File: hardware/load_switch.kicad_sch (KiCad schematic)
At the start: 24 parts, among them Q1 IPT015N10N5, Q2 IPT015N10N5, Q3 IPT015N10N5, Q4 IPT015N10N5, Q5 IPT015N10N5, Q6 IPT015N10N5, Q7 IPT015N10N5, Q8 IPT015N10N5

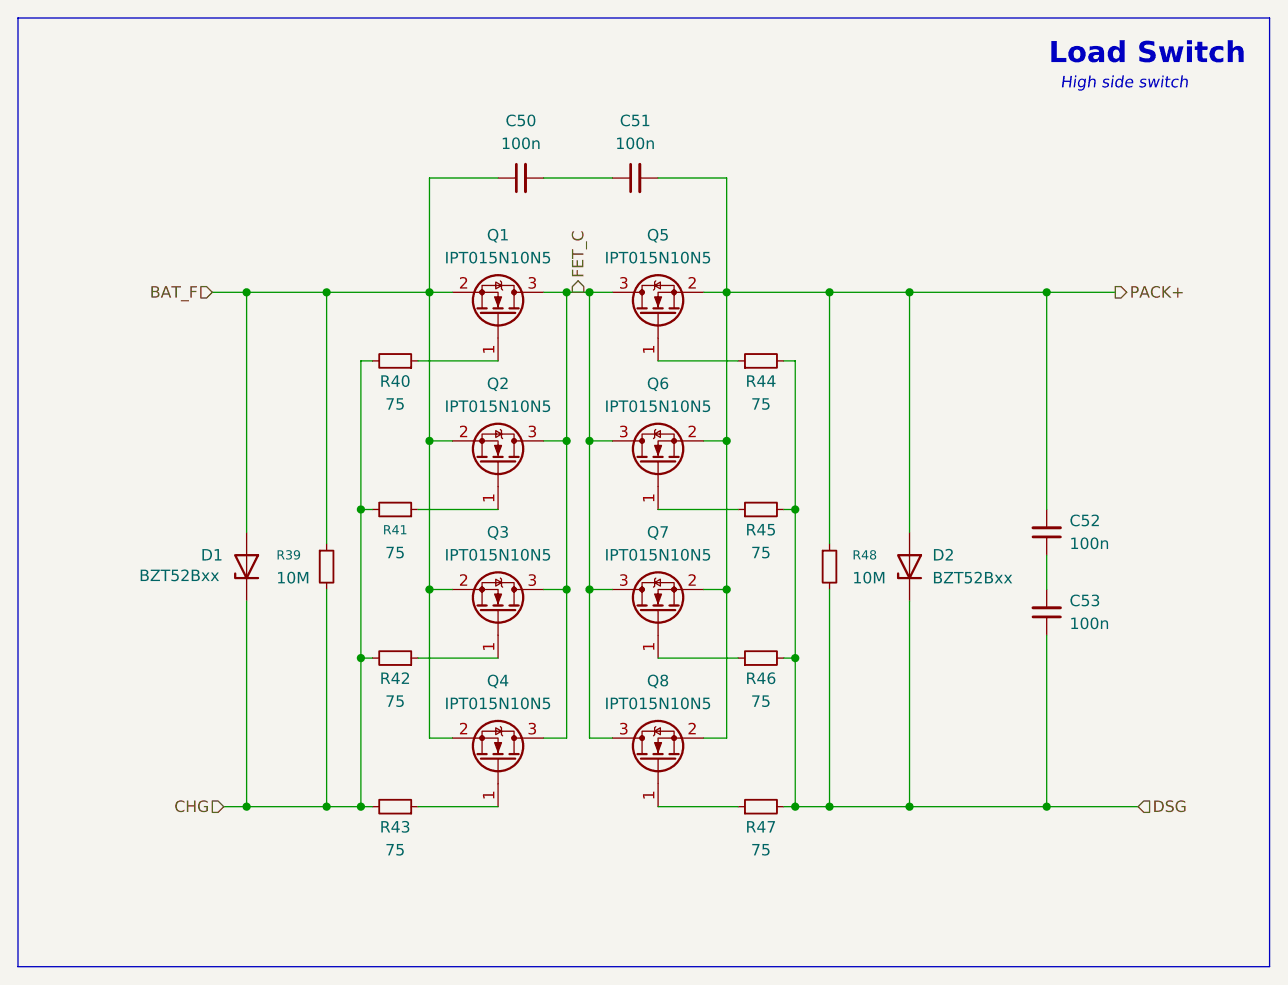
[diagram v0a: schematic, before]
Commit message: Majority of layout placement done
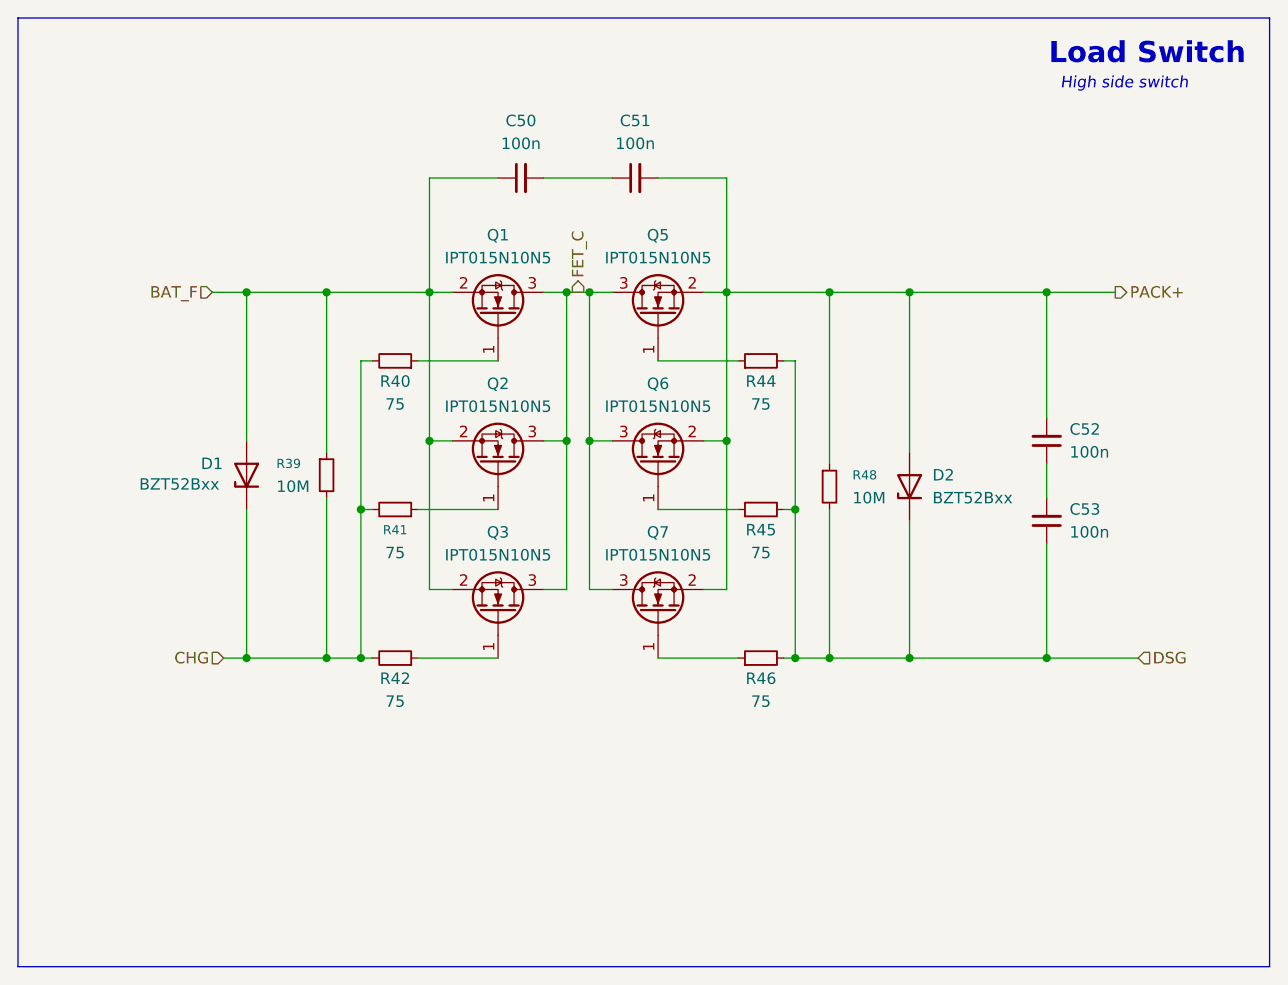
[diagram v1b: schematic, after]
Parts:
- removed Q4, Q8: IPT015N10N5, Package_TO_SOT_SMD:Infineon_PG-HSOF-8-1_ThermalVias, symbol Transistor_FET:IPT015N10N5
- removed R43, R47: 75, Capacitor_SMD:C_0603_1608Metric, symbol Device:R_Small
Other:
- moved on the sheet: C52, C53, D1, D2, R39, R48

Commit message: First Layout placement
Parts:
- R40, R41, R42, R44, R45, R46: footprint Capacitor_SMD:C_0603_1608Metric -> Capacitor_SMD:C_0402_1005Metric
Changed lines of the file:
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@@
 			)
 		)
-		(property "Footprint" "Capacitor_SMD:C_0603_1608Metric"
+		(property "Footprint" "Capacitor_SMD:C_0402_1005Metric"
 			(at 156.21 113.03 0)
 			(effects
@@
 			)
 		)
-		(property "Footprint" "Capacitor_SMD:C_0603_1608Metric"
+		(property "Footprint" "Capacitor_SMD:C_0402_1005Metric"
 			(at 115.57 96.52 0)
 			(effects
@@
 			)
 		)
-		(property "Footprint" "Capacitor_SMD:C_0603_1608Metric"
+		(property "Footprint" "Capacitor_SMD:C_0402_1005Metric"
 			(at 115.57 80.01 0)
 			(effects
@@
 			)
 		)
-		(property "Footprint" "Capacitor_SMD:C_0603_1608Metric"
+		(property "Footprint" "Capacitor_SMD:C_0402_1005Metric"
 			(at 115.57 113.03 0)
 			(effects
@@
 			)
 		)
-		(property "Footprint" "Capacitor_SMD:C_0603_1608Metric"
+		(property "Footprint" "Capacitor_SMD:C_0402_1005Metric"
 			(at 156.21 80.01 0)
 			(effects
@@
 			)
 		)
-		(property "Footprint" "Capacitor_SMD:C_0603_1608Metric"
+		(property "Footprint" "Capacitor_SMD:C_0402_1005Metric"
 			(at 156.21 96.52 0)
 			(effects

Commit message: Remove U.fL connector and improve layout
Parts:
- Q1: Alternate C2979263 -> (none)
- Q2, Q3, Q5, Q6, Q7: Alternate C2979263 -> (none); Notes (none) -> Alternative: C2979263
